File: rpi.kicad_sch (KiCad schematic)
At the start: 40 parts, among them J1 Conn_02x08_Counter_Clockwise_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, J101 Conn_01x03_Pin, J4 Conn_01x04_Pin, J5 Conn_02x08_Counter_Clockwise_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, J6 2169890001, U3 RASPBERRY_PI_ZERO_2_W

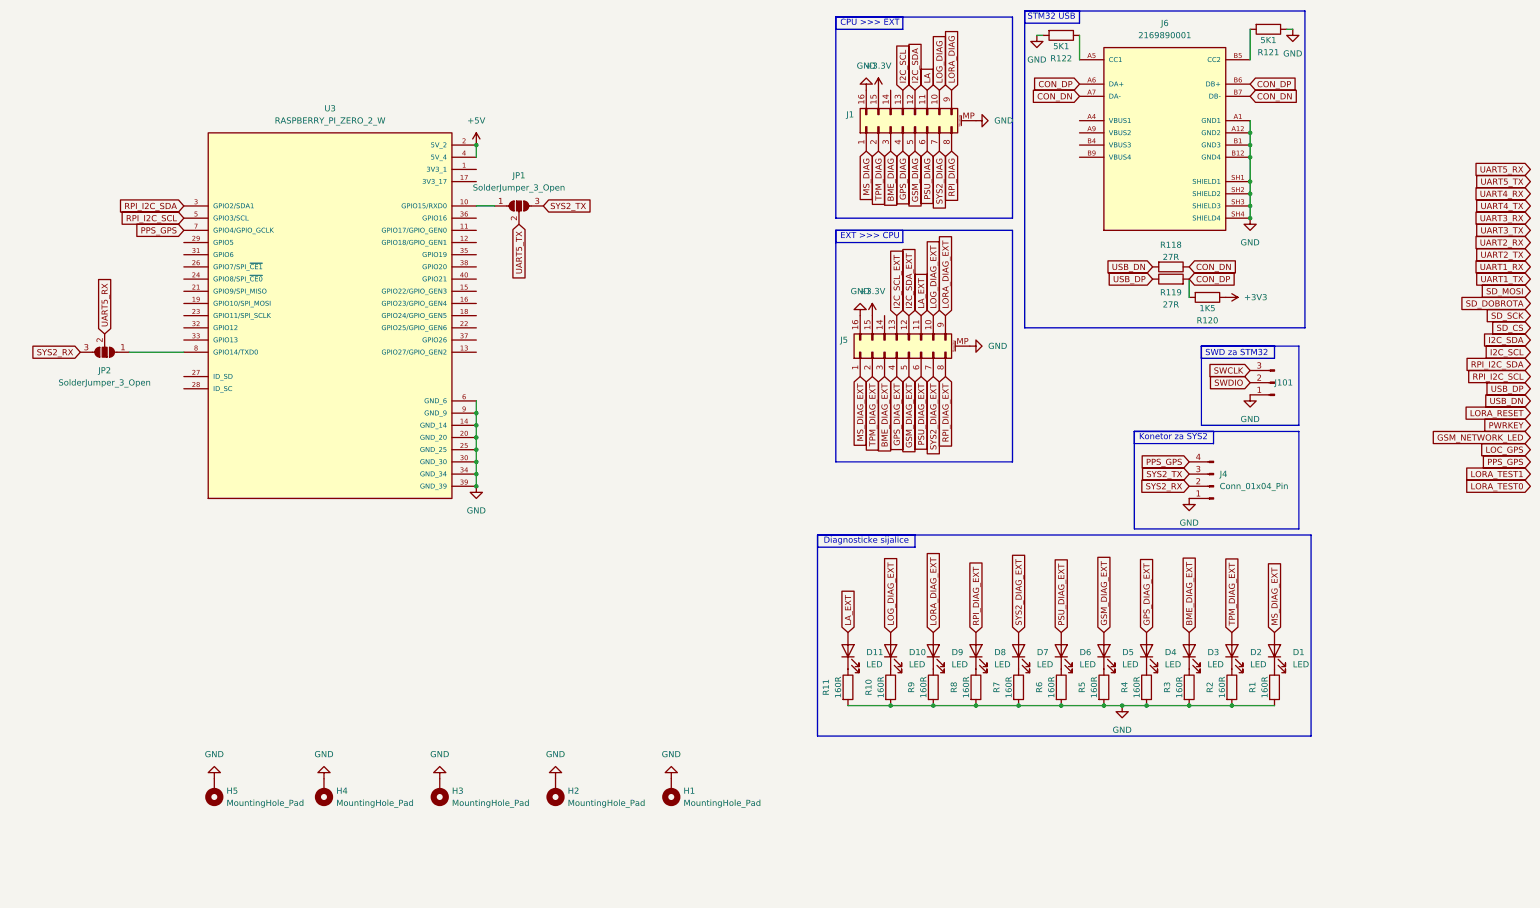
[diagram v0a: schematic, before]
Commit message: Napajanje
David i njegova biblioteka su pravili probleme
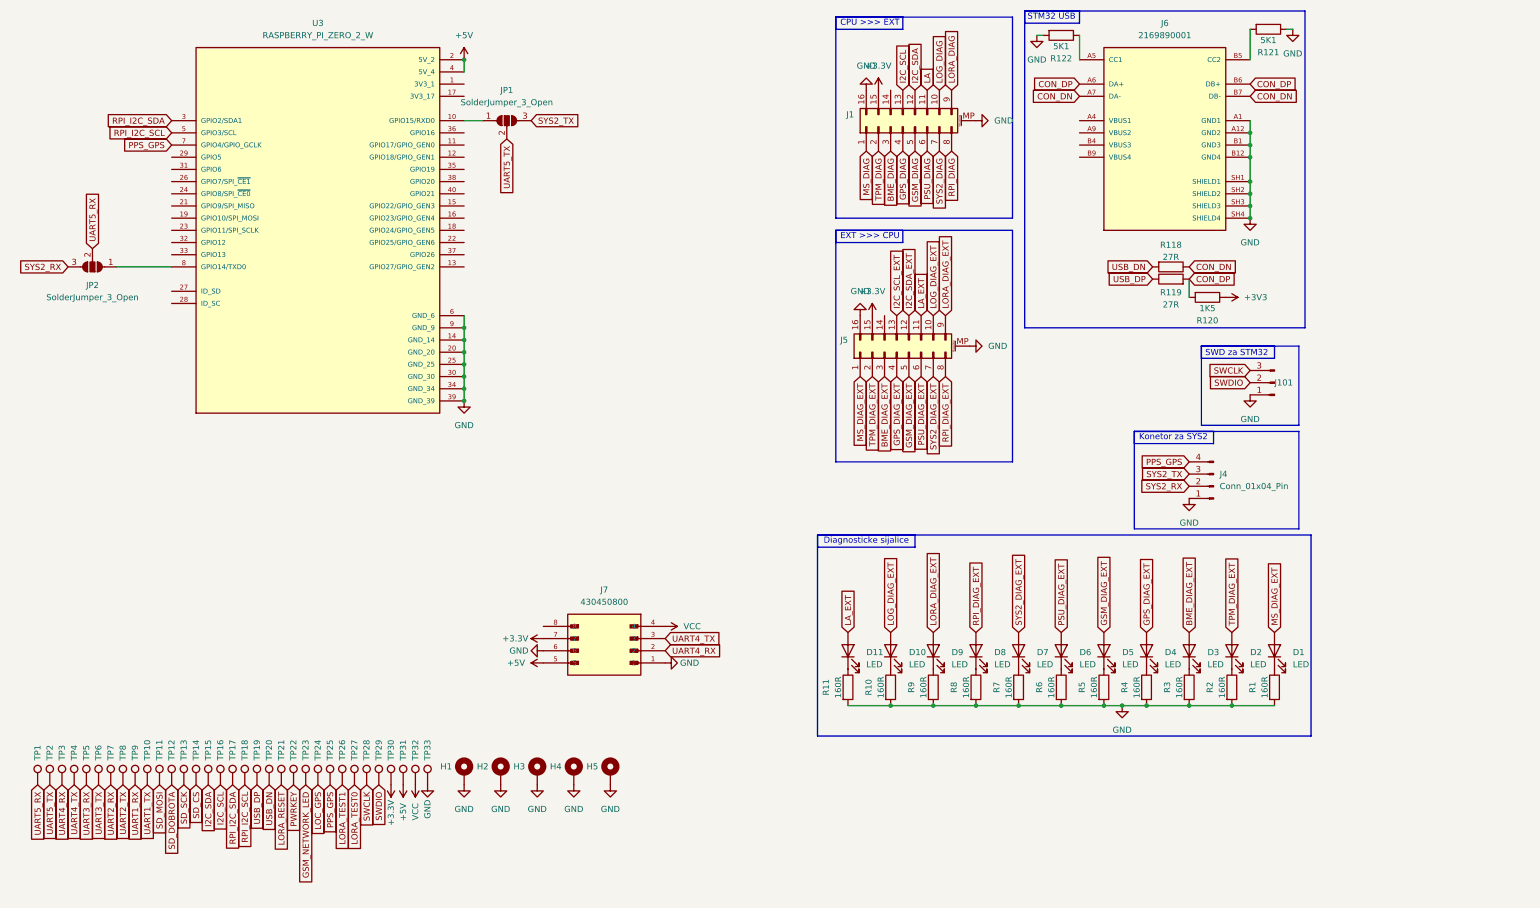
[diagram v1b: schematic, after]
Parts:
- added J7: 430450800, 430450800:MOLEX_430450800, symbol 430450800:430450800
- added TP1, TP10, TP11, TP12, TP13, TP14, TP15, TP16, TP17, TP18, TP19, TP2, TP20, TP21, TP22, TP23, TP24, TP25, TP26, TP27, TP28, TP29, TP3, TP30, TP31, TP32, TP33, TP4, TP5, TP6, TP7, TP8, TP9: TestPoint, TestPoint:TestPoint_Pad_D1.0mm, symbol Connector:TestPoint
- renumbered H5 to H1, H1 to H5
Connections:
- net +3.3V: now also J7.7, TP30.1
- net +5V: now also J7.5, TP31.1
- net GND: now also J7.1, J7.6, TP33.1
- net GSM_NETWORK_LED: now also TP23.1
- net I2C_SCL: now also TP16.1
- net I2C_SDA: now also TP15.1
- net LOC_GPS: now also TP24.1
- net LORA_RESET: now also TP21.1
- net LORA_TEST0: now also TP27.1
- net LORA_TEST1: now also TP26.1
- net PPS_GPS: now also TP25.1
- net PWRKEY: now also TP22.1
- net RPI_I2C_SCL: now also TP18.1
- net RPI_I2C_SDA: now also TP17.1
- net SD_CS: now also TP14.1
- net SD_DOBROTA: now also TP12.1
- net SD_MOSI: now also TP11.1
- net SD_SCK: now also TP13.1
- net SWCLK: now also TP28.1
- net SWDIO: now also TP29.1
- net UART1_RX: now also TP9.1
- net UART1_TX: now also TP10.1
- net UART2_RX: now also TP7.1
- net UART2_TX: now also TP8.1
- net UART3_RX: now also TP5.1
- net UART3_TX: now also TP6.1
- net UART4_RX: now also J7.2, TP3.1
- net UART4_TX: now also J7.3, TP4.1
- net UART5_RX: now also TP1.1
- net UART5_TX: now also TP2.1
- net USB_DN: now also TP20.1
- net USB_DP: now also TP19.1
- new net VCC: J7.4, TP32.1
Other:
- moved on the sheet: H1, H2, H3, H4, H5, JP1, JP2, U3
